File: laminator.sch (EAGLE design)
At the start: 19 parts, among them T1 BT138-H

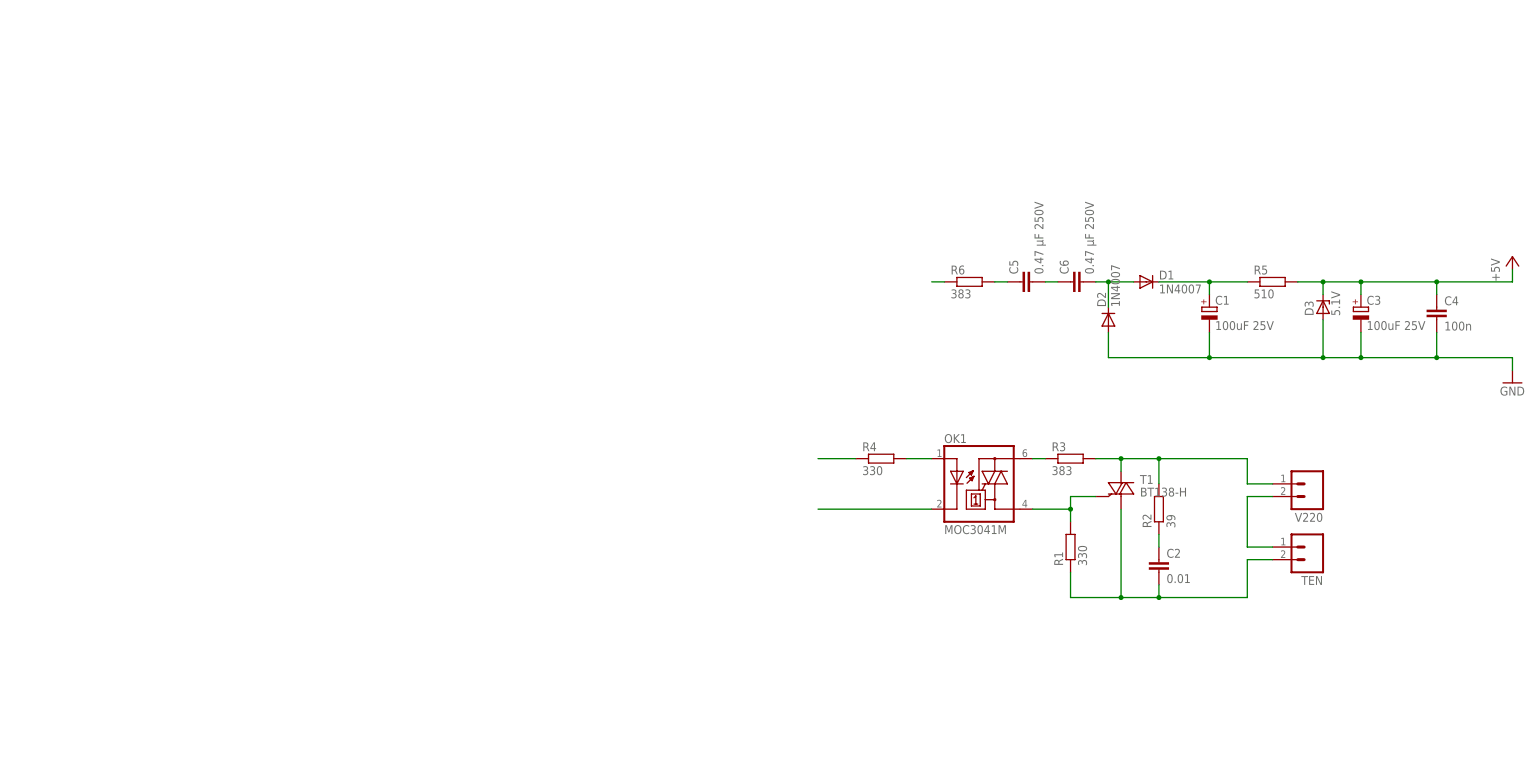
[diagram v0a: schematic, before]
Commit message: layout changes
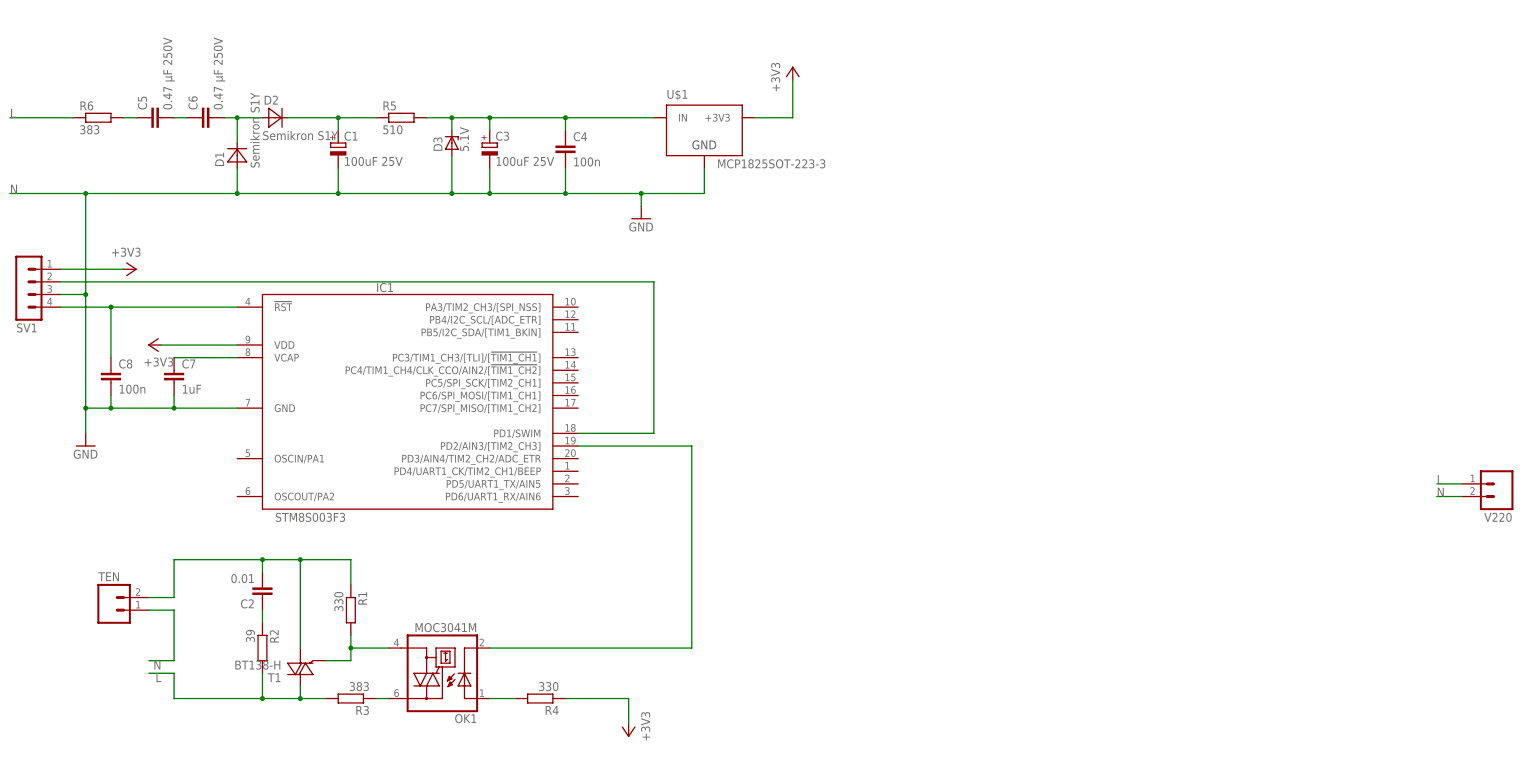
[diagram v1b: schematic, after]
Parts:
- added C7: 1uF, rcl:C-EUC0805
- added C8: 100n, rcl:C-EUC0805
- added IC1: STM8S003F3, stm8:STM8S003F3
- added SV1: (no value), con-lstb:MA04-1
- added U$1: MCP1825SOT-223-3, SteelCaveRobotics-Power:MCP1825SOT-223-3
- D1, D2: value 1N4007 -> Semikron S1Y; device diode:1N4004 -> diode:MBRA340T3
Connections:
- removed net +5V: C3.+, C4.1, D3.C, R5.2
- removed net GND: C1.-, C3.-, C4.2, D2.A, D3.A
- removed net N$13: R6.1
- new net +3V3: IC1.VDD, R4.1, SV1.1, U$1.+3V3
- new net L: R2.2, R3.2, R6.1, T1.A2, V220.1
- new net N: C1.-, C3.-, C4.2, C7.2, C8.2, D1.A, D3.A, IC1.GND, SV1.3, TEN.1, U$1.GND@2, V220.2
- new net N$12: C3.+, C4.1, D3.C, R5.2, U$1.IN
- net N$10: now also IC1.PD2/AIN3/[TIM2_CH3]
- net N$11: now also D2.C; no longer D1.C
- net N$2: now also C7.1, IC1.VCAP; no longer R2.2, R3.2, T1.A2, V220.1
- net N$5: now also D1.C, D2.A; no longer D1.A, D2.C
- net N$7: now also C8.1, IC1.!RST, SV1.4; no longer TEN.1, V220.2
- net N$9: now also IC1.PD1/SWIM, SV1.2; no longer R4.1
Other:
- moved on the sheet: C1, C2, C3, C4, C5, C6, D3, OK1, R1, R2, R3, R4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
